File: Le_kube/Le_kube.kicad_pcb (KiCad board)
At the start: 2 copper layers, 52 x 125 mm, 50 parts, among them J1 Conn_01x06_Male, J2 USB_A, J3 Barrel_Jack_Switch, Q1 IRLB8721PBF, SW1 I/O, SW2 RST, SW3 SW_Push, SW4 SW_Push, SW5 SW_Push, U0 ATmega328PB-AU, U1 LM75A, U2 128x64_OLED, U3 TLC555CDR, U4 ESP8266-01_ESP-01, Y1 Crystal

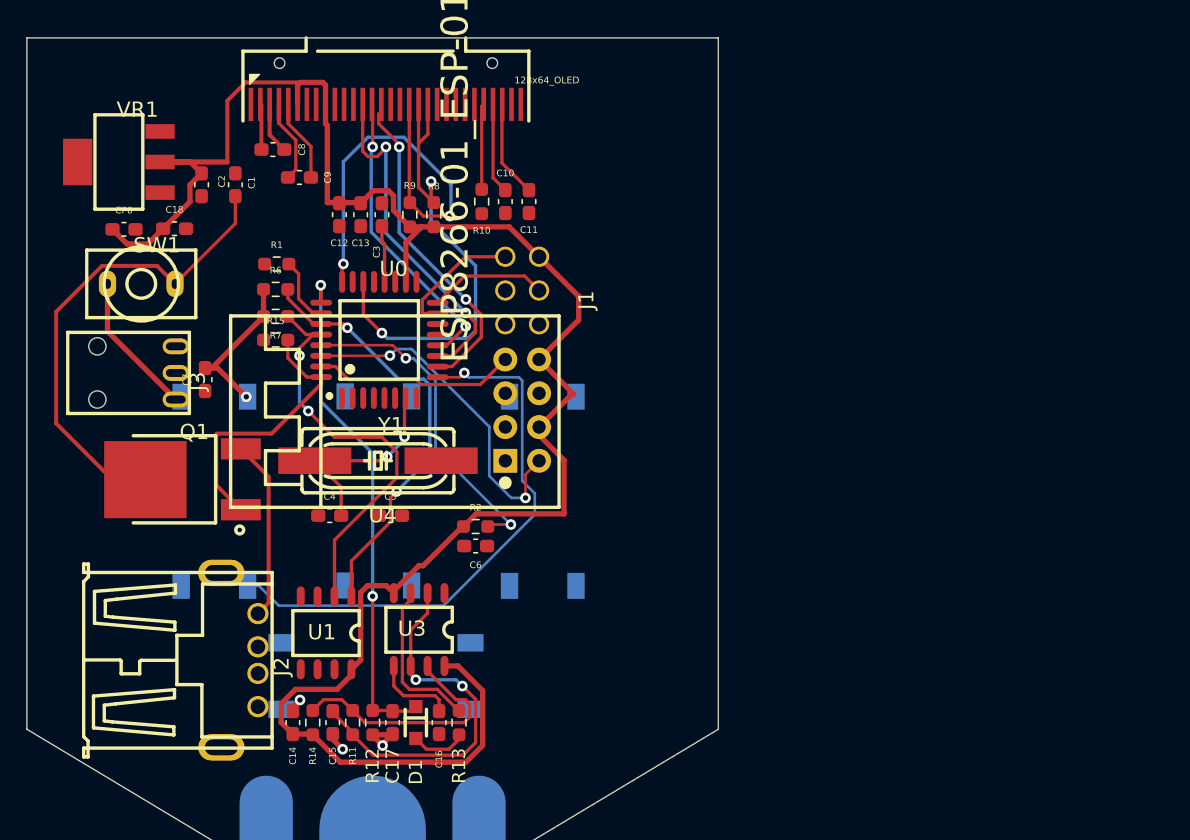
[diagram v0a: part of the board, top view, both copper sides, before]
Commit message: debut du routage (commit de secours)
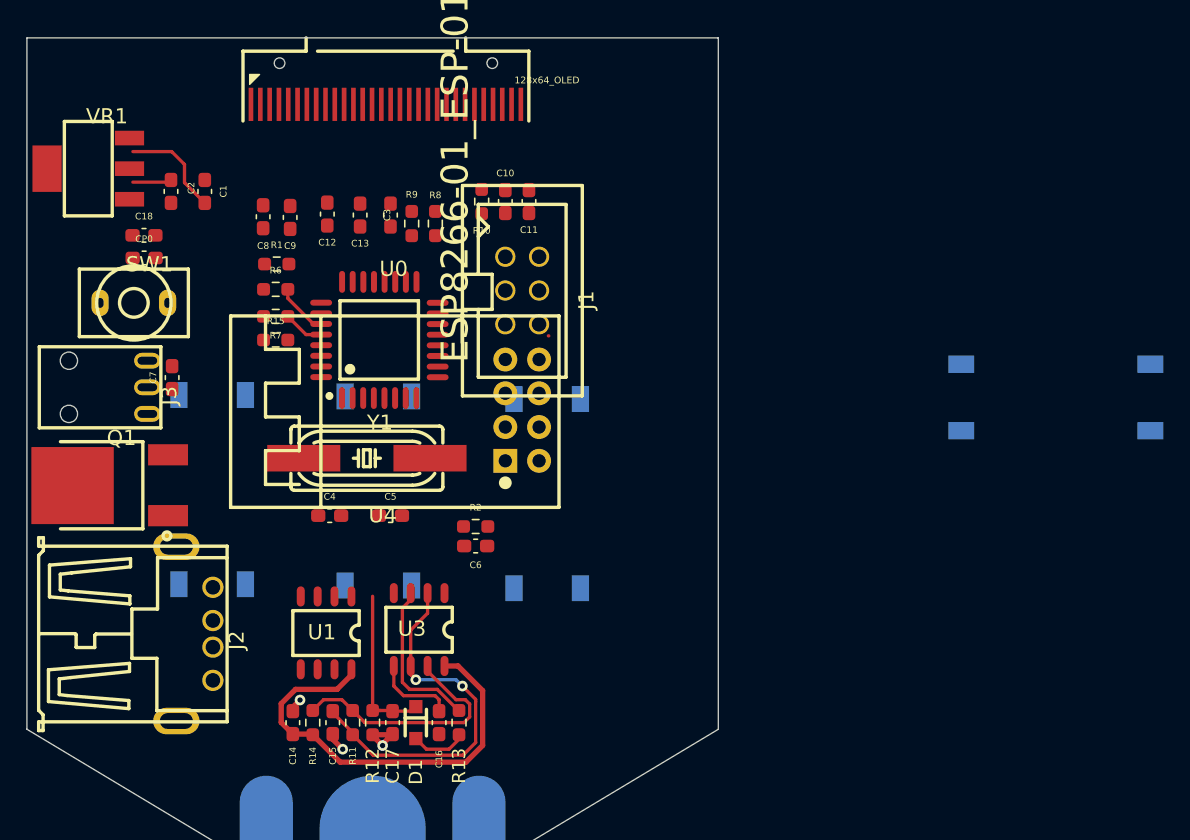
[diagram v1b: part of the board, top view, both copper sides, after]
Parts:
- moved SW2 55.3 mm to (151.4, 82.0)
- moved Q1 5.49 mm to (81.0, 88.6)
- moved C8 5.11 mm to (91.8, 68.5), turned to 270 degrees
- moved J2 3.92 mm to (86.6, 99.8)
- moved C9 3.09 mm to (93.8, 68.5), turned to 270 degrees
- moved CP0 2.63 mm to (82.8, 71.6)
- moved C7 2.48 mm to (84.9, 80.5)
- moved J3 2.40 mm to (83.1, 81.3)
- moved C1 2.35 mm to (87.4, 66.5)
- moved C18 2.35 mm to (82.8, 69.8)
- moved C2 2.35 mm to (84.8, 66.5)
- moved VR1 2.35 mm to (78.6, 64.8)
- moved SW1 1.54 mm to (82.0, 74.9)
- moved C12 0.91 mm to (96.6, 68.3)
- moved Y1 0.85 mm to (99.6, 86.6)
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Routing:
- net +3V3: track 160.8 -> 35.4 mm, vias 1 -> 0
- net Net-(R5-Pad2): track 42.2 -> 0.00 mm, vias 1 -> 0
- net /SCREEN_MISO: track 37.3 -> 0.00 mm, vias 2 -> 0
- net /SCREEN_SCK: track 32.6 -> 0.00 mm, vias 2 -> 0
- net Net-(C1-Pad2): track 36.3 -> 7.81 mm
- net /SDA: track 32.4 -> 3.98 mm, vias 2 -> 0
- net /SCL: track 30.9 -> 3.07 mm, vias 2 -> 0
- net /HUM: track 39.1 -> 12.7 mm, vias 2 -> 0
- net /SCREEN_SS: track 26.1 -> 0.00 mm, vias 2 -> 0
- net /ESP_TX: track 25.6 -> 0.00 mm, vias 2 -> 0
- net /SCREEN_MOSI: track 25.0 -> 0.00 mm, vias 2 -> 0
- net Net-(C6-Pad2): track 24.7 -> 0.00 mm, vias 2 -> 0
- net /SCREEN_RST: track 22.4 -> 0.00 mm, vias 2 -> 0
- net Net-(Q1-Pad1): track 20.9 -> 0.00 mm
- net Net-(C4-Pad2): track 15.5 -> 0.00 mm, vias 2 -> 0
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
